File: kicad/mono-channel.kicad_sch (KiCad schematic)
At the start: 12 parts, among them U1 TL072

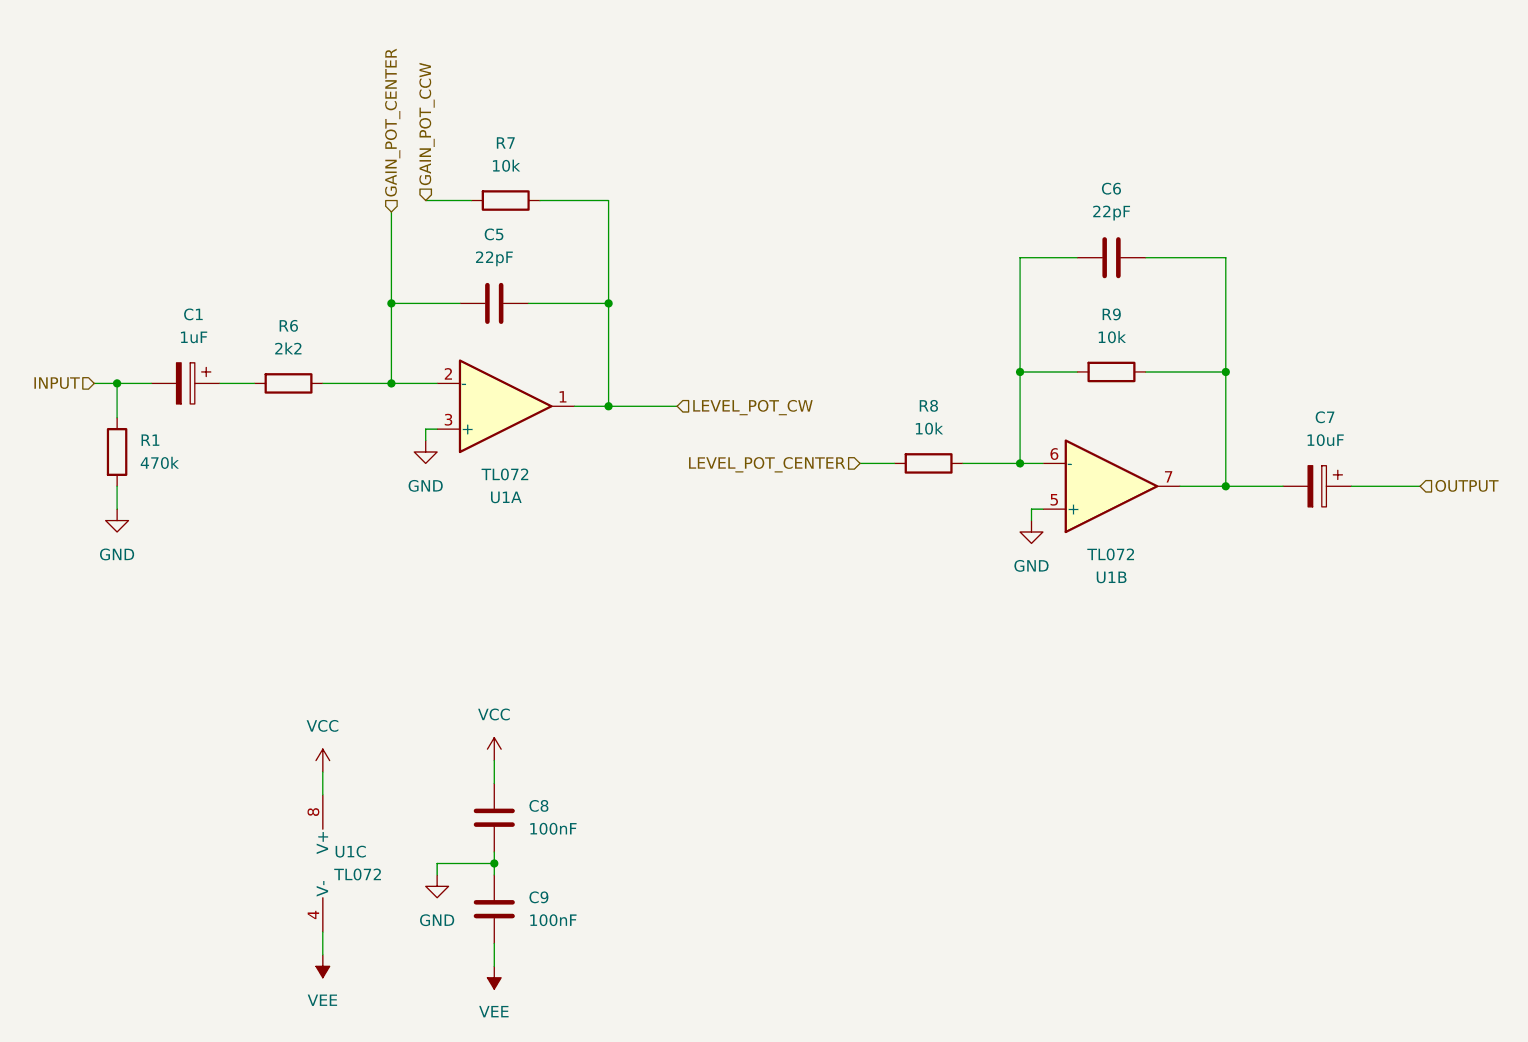
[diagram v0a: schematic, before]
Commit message: Updating everything and adding gerbers
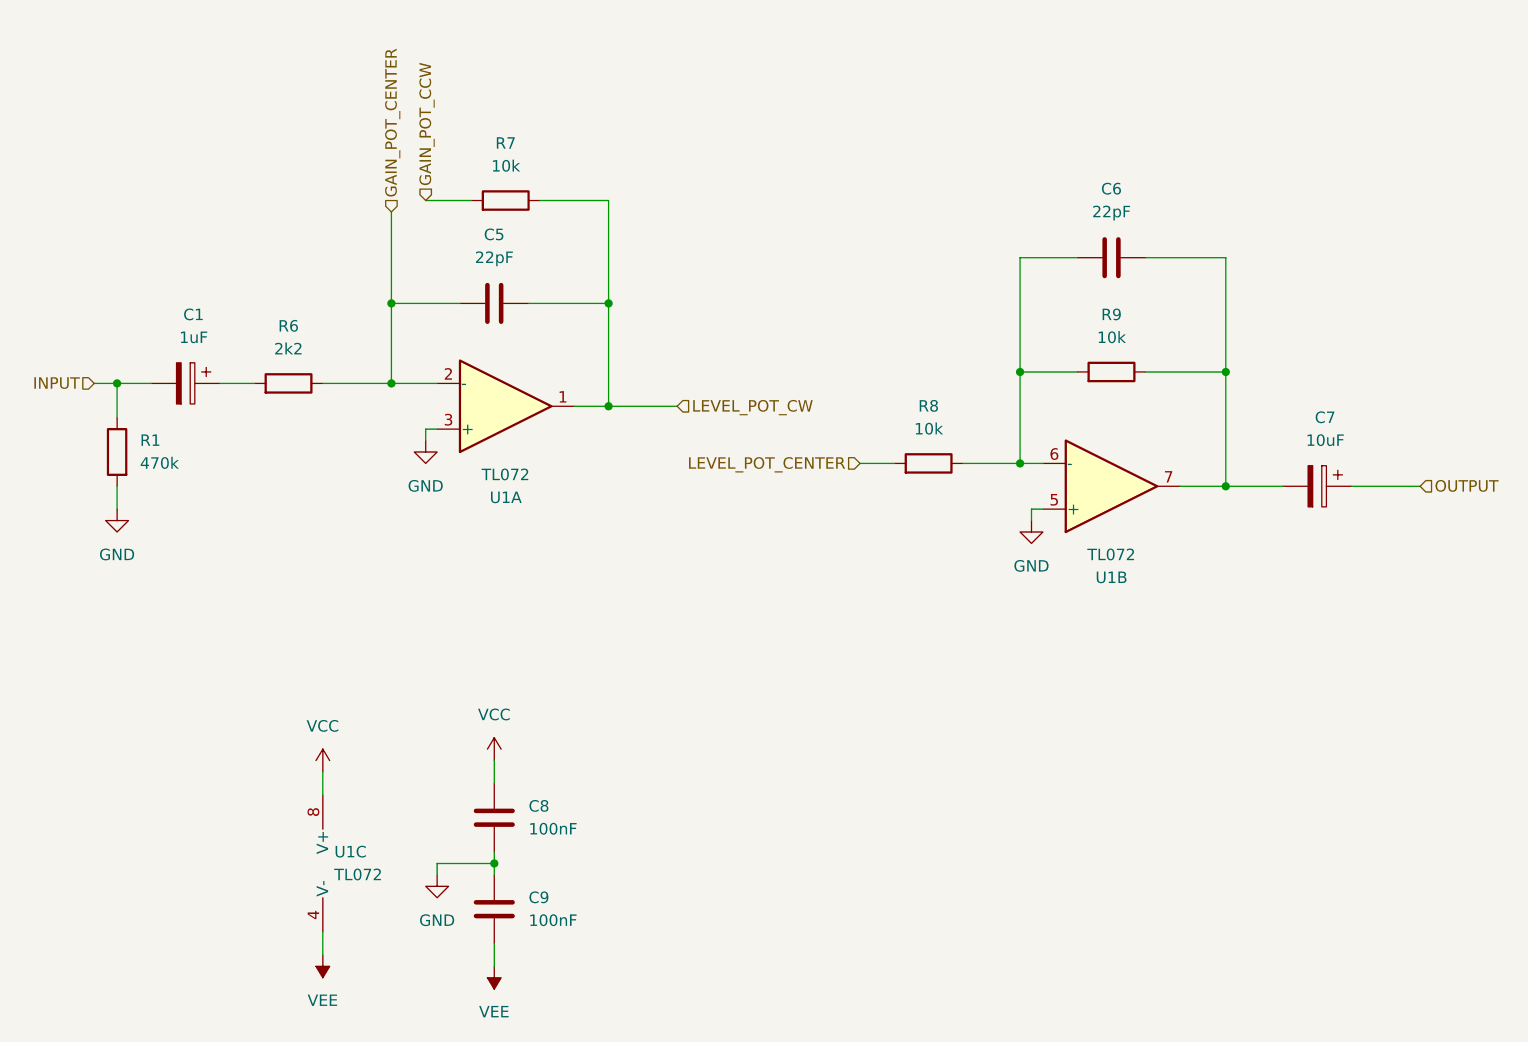
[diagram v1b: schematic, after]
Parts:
- C1, C7: footprint Capacitor_THT:CP_Radial_D5.0mm_P2.00mm -> Rumblesan_Standard_Parts:CP_Radial_D5.0mm_P2.00mm; symbol Standard_Parts:C_Polarized -> Rumblesan_Standard_Parts:C_Polarized
- C5, C6, C8, C9: symbol Standard_Parts:C -> Rumblesan_Standard_Parts:C
- R1, R6, R7, R8, R9: symbol Standard_Parts:R -> Rumblesan_Standard_Parts:R
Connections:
- net GAIN_POT_CCW: now also R7.1; no longer R7.2
- net GAIN_POT_CENTER: now also R6.2; no longer R6.1
- net GND: now also R1.1; no longer R1.2
- net INPUT: now also R1.2; no longer R1.1
- net LEVEL_POT_CENTER: now also R8.1; no longer R8.2
- net LEVEL_POT_CW: now also R7.2; no longer R7.1
- net at C6.2, C7.2, U1.7: now also R9.2; no longer R9.1
- net at C6.1, U1.6 (-): now also R8.2, R9.1; no longer R8.1, R9.2
- net at C1.1: now also R6.1; no longer R6.2
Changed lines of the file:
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@@
 	)
 	(symbol
-		(lib_id "Standard_Parts:C")
+		(lib_id "Rumblesan_Standard_Parts:C")
 		(at 92.71 68.58 90)
 		(unit 1)
@@
 	)
 	(symbol
-		(lib_id "Standard_Parts:C_Polarized")
+		(lib_id "Rumblesan_Standard_Parts:C_Polarized")
 		(at 184.15 88.9 270)
 		(unit 1)
@@
 			)
 		)
-		(property "Footprint" "Capacitor_THT:CP_Radial_D5.0mm_P2.00mm"
+		(property "Footprint" "Rumblesan_Standard_Parts:CP_Radial_D5.0mm_P2.00mm"
 			(at 184.15 95.25 90)
 			(effects
@@
 	)
 	(symbol
-		(lib_id "Standard_Parts:C")
+		(lib_id "Rumblesan_Standard_Parts:C")
 		(at 161.29 63.5 90)
 		(unit 1)
@@
 	)
 	(symbol
-		(lib_id "Standard_Parts:C")
+		(lib_id "Rumblesan_Standard_Parts:C")
 		(at 92.71 125.73 180)
 		(unit 1)
@@
 	)
 	(symbol
-		(lib_id "Standard_Parts:R")
+		(lib_id "Rumblesan_Standard_Parts:R")
 		(at 140.97 86.36 90)
 		(unit 1)
@@
 	)
 	(symbol
-		(lib_id "Standard_Parts:C_Polarized")
+		(lib_id "Rumblesan_Standard_Parts:C_Polarized")
 		(at 58.42 77.47 270)
 		(unit 1)
@@
 			)
 		)
-		(property "Footprint" "Capacitor_THT:CP_Radial_D5.0mm_P2.00mm"
+		(property "Footprint" "Rumblesan_Standard_Parts:CP_Radial_D5.0mm_P2.00mm"
 			(at 58.42 83.82 90)
 			(effects
@@
 	)
 	(symbol
-		(lib_id "Standard_Parts:R")
+		(lib_id "Rumblesan_Standard_Parts:R")
 		(at 69.85 77.47 90)
 		(unit 1)
@@
 	)
 	(symbol
-		(lib_id "Standard_Parts:R")
+		(lib_id "Rumblesan_Standard_Parts:R")
 		(at 161.29 76.2 90)
 		(unit 1)
@@
 	)
 	(symbol
-		(lib_id "Standard_Parts:C")
+		(lib_id "Rumblesan_Standard_Parts:C")
 		(at 92.71 135.89 180)
 		(unit 1)
@@
 	)
 	(symbol
-		(lib_id "Standard_Parts:R")
+		(lib_id "Rumblesan_Standard_Parts:R")
 		(at 93.98 57.15 90)
 		(unit 1)
@@
 	)
 	(symbol
-		(lib_id "Standard_Parts:R")
+		(lib_id "Rumblesan_Standard_Parts:R")
 		(at 50.8 85.09 180)
 		(unit 1)
